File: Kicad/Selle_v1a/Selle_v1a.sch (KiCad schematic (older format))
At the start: 13 parts

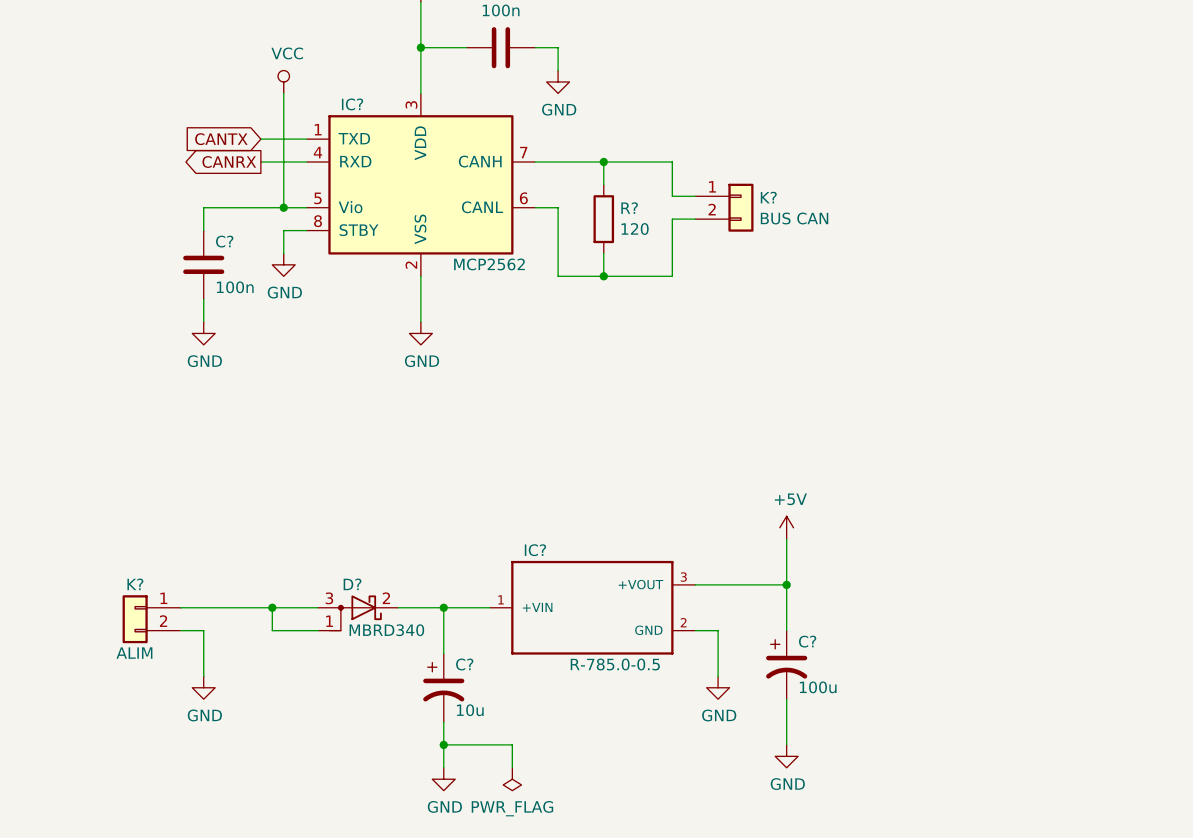
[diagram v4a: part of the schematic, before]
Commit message: Update
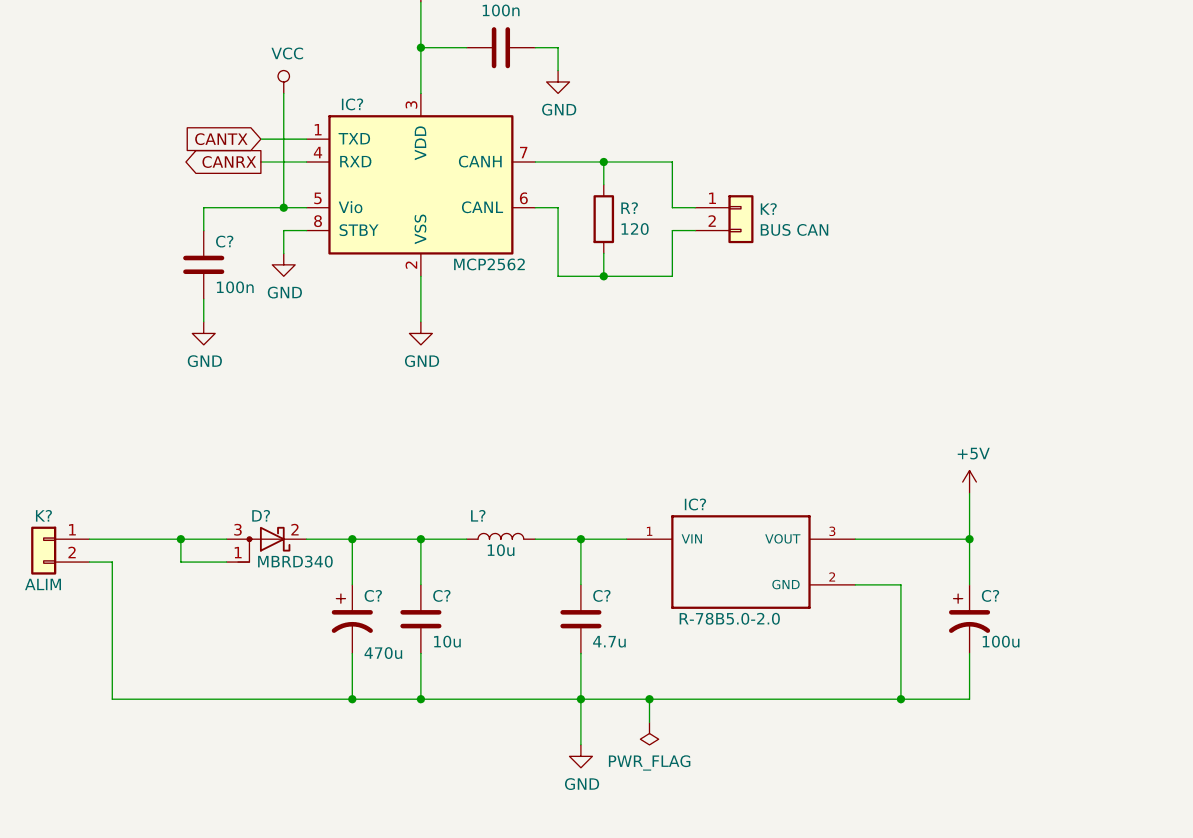
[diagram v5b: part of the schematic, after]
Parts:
- removed C?: 10u, symbol Device:CP1
- removed IC?: R-785.0-0.5, RECOM_R-785.0-0.5, symbol R-785.0-0.5:R-785.0-0.5
- added C?: 4.7u, symbol Device:C
- added C?: 10u, symbol Device:C
- added C?: 470u, symbol Device:CP1
- added IC?: R-78B5.0-2.0, CONV_R-78B15-2.0, symbol R-78B15-2.0:R-78B15-2.0
- added L?: 10u, symbol Device:L
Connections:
- net +5V: now also IC?.3 (VOUT)
- net GND: now also C?.2, C?.2, C?.2, IC?.2 (GND)
- net at D?.2 (K): now also C?.1, C?.1, L?.1
- new net: C?.1, IC?.1 (VIN), L?.2
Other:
- moved on the sheet: C?, D?, K?

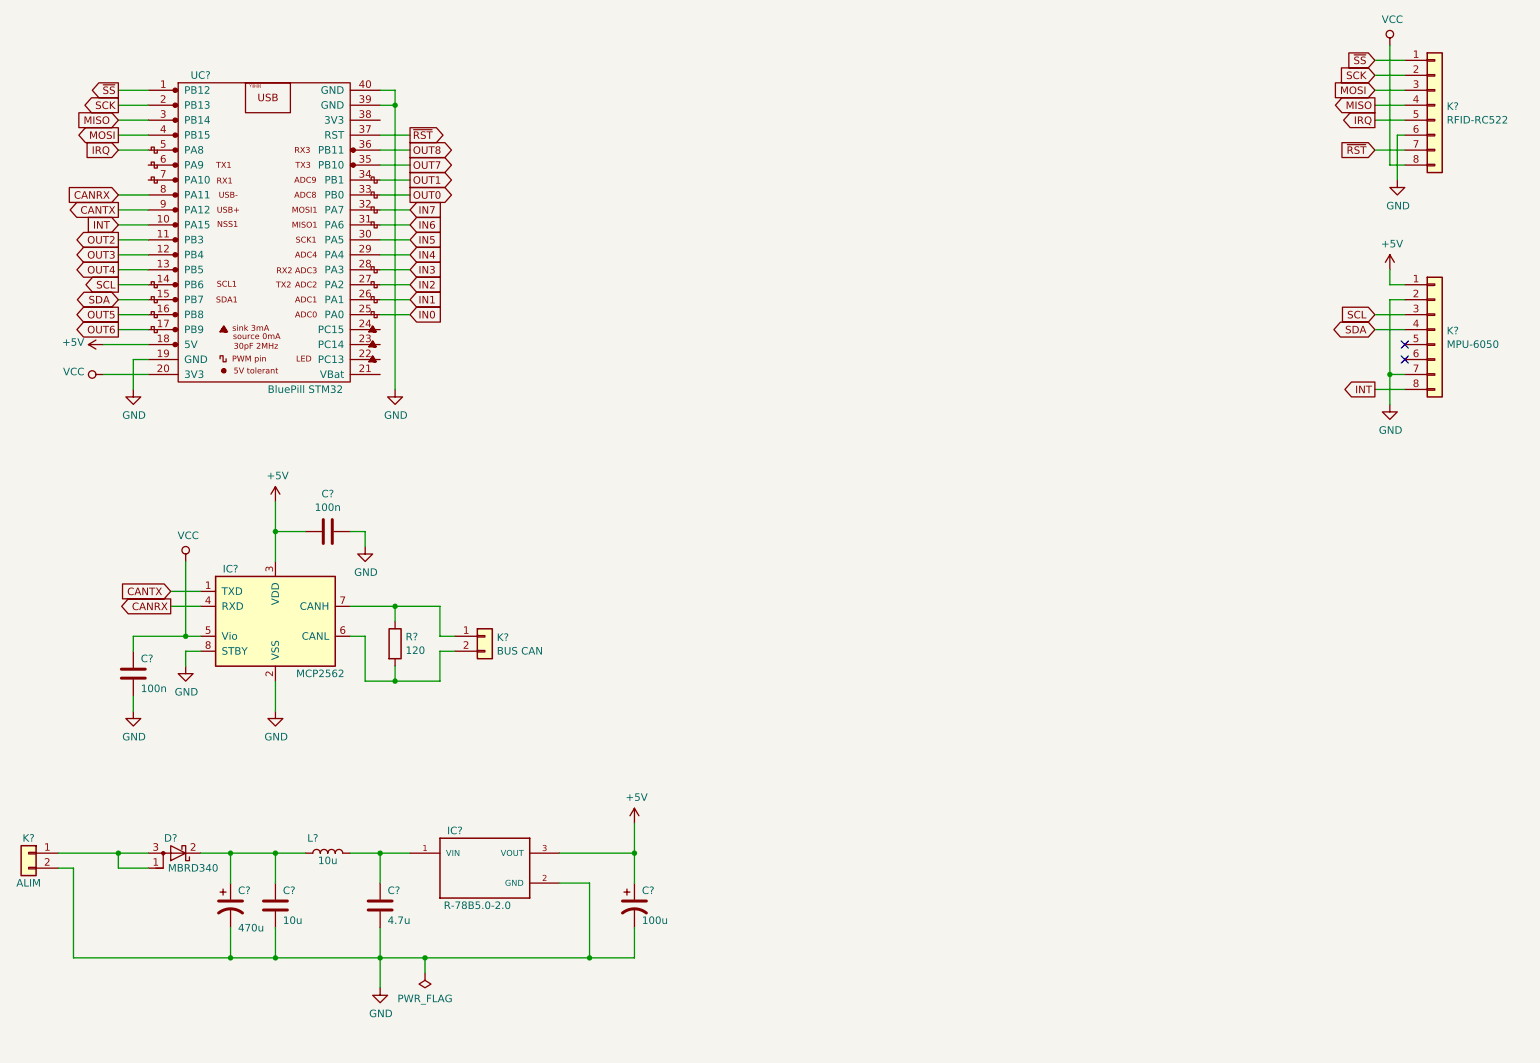
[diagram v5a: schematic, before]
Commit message: Update
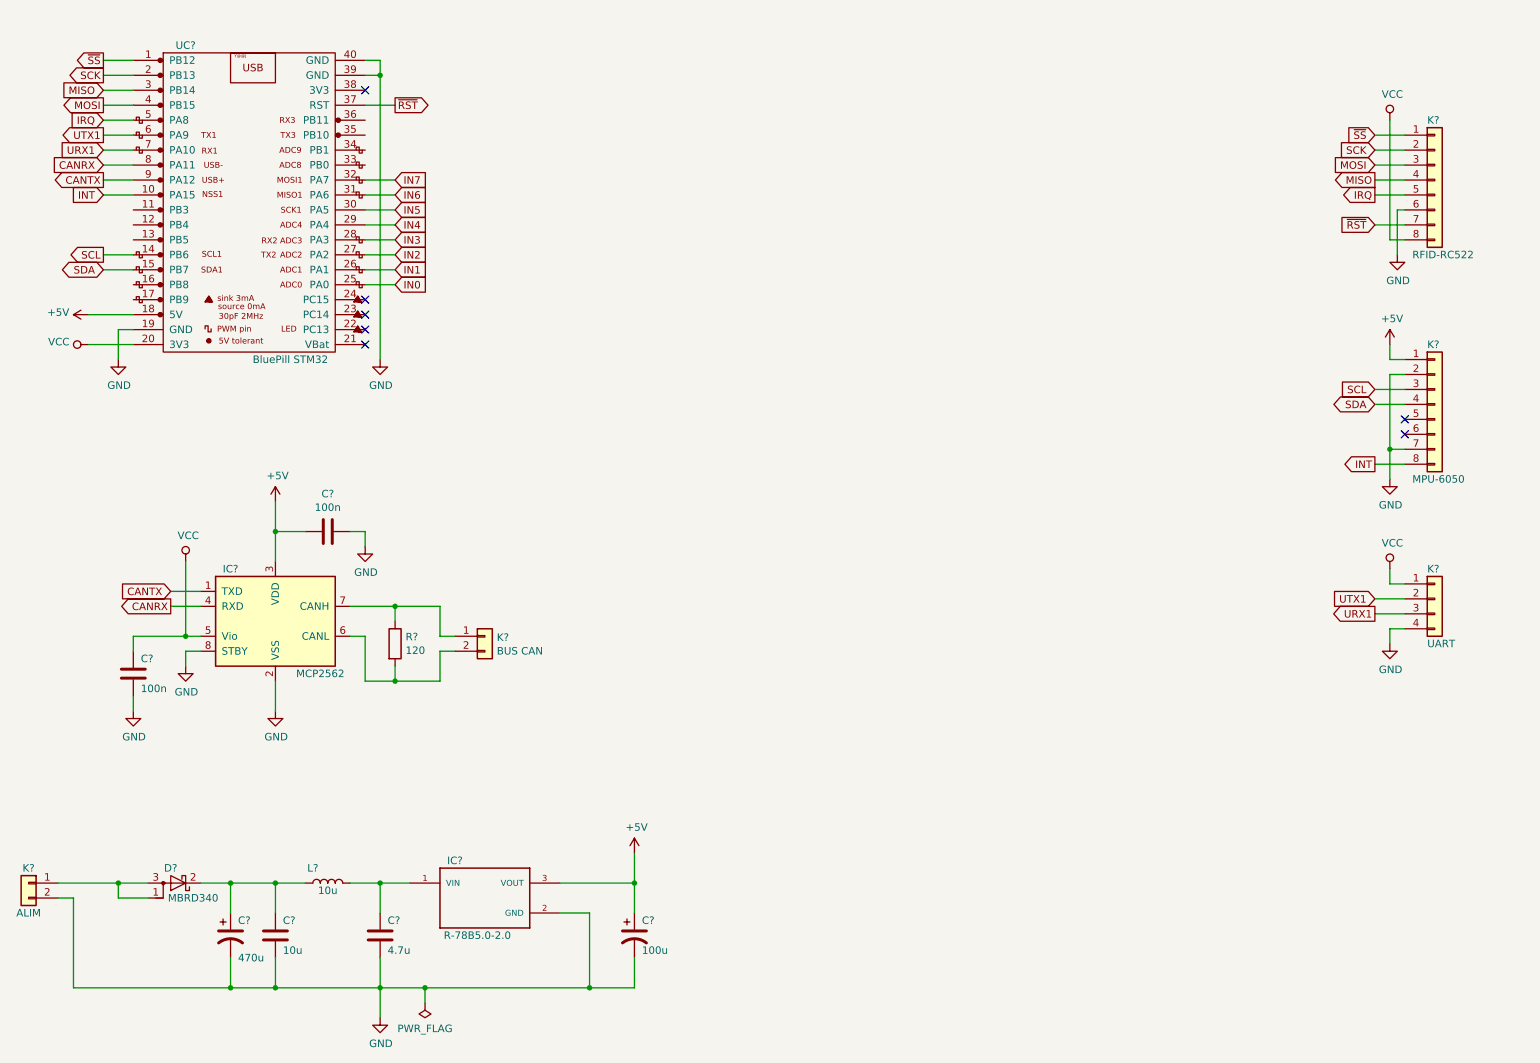
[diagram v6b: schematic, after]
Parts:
- added K?: UART, symbol Connector_Generic:Conn_01x04
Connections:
- net GND: now also K?.4 (Pin_4)
- net VCC: now also K?.1 (Pin_1)
- net UTX1: now reaches UC?.6 (PA9)
- net UTX1: now also K?.2 (Pin_2)
- net URX1: now reaches UC?.7 (PA10)
- net URX1: now also K?.3 (Pin_3)
- net OUT0: no longer names the net of UC?.33 (PB0)
- net OUT1: no longer names the net of UC?.34 (PB1)
- net OUT2: no longer names the net of UC?.11 (PB3)
- net OUT3: no longer names the net of UC?.12 (PB4)
- net OUT4: no longer names the net of UC?.13 (PB5)
- net OUT5: no longer names the net of UC?.16 (PB8)
- net OUT6: no longer names the net of UC?.17 (PB9)
- net OUT7: no longer names the net of UC?.35 (PB10)
- net OUT8: no longer names the net of UC?.36 (PB11)
- no-connect marks 2 -> 7
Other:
- moved on the sheet: C?, D?, IC?, K?, L?, UC?

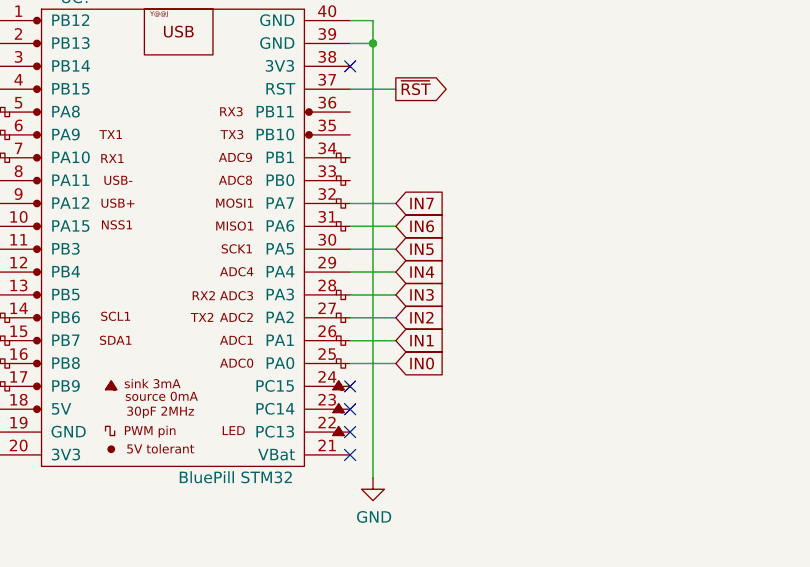
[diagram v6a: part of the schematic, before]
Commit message: Update
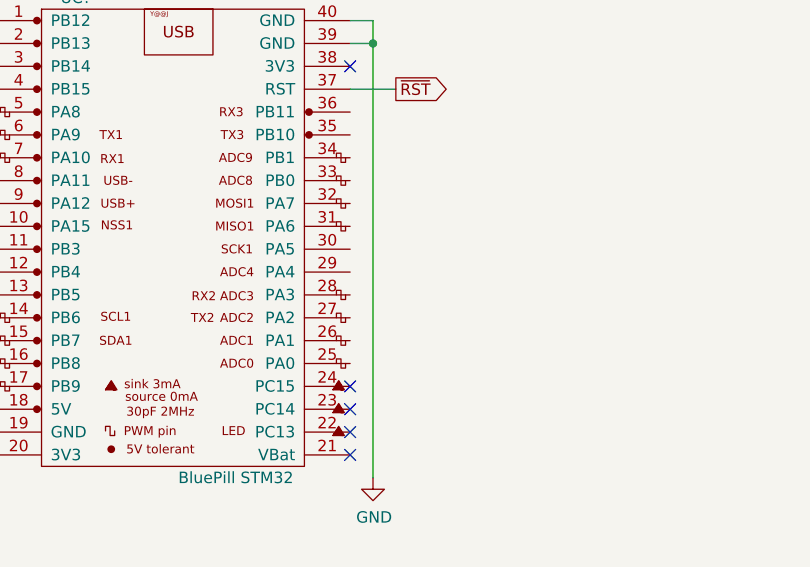
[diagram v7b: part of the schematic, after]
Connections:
- net IN0: no longer names the net of UC?.25 (PA0)
- net IN1: no longer names the net of UC?.26 (PA1)
- net IN2: no longer names the net of UC?.27 (PA2)
- net IN3: no longer names the net of UC?.28 (PA3)
- net IN4: no longer names the net of UC?.29 (PA4)
- net IN5: no longer names the net of UC?.30 (PA5)
- net IN6: no longer names the net of UC?.31 (PA6)
- net IN7: no longer names the net of UC?.32 (PA7)
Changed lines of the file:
@@
 NoConn ~ 3050 2900
 NoConn ~ 3050 1200
-Text GLabel 3250 1800 2    50   Input ~ 0
-IN7
-Text GLabel 3250 1900 2    50   Input ~ 0
-IN6
-Text GLabel 3250 2000 2    50   Input ~ 0
-IN5
-Text GLabel 3250 2100 2    50   Input ~ 0
-IN4
-Text GLabel 3250 2200 2    50   Input ~ 0
-IN3
-Text GLabel 3250 2300 2    50   Input ~ 0
-IN2
-Text GLabel 3250 2400 2    50   Input ~ 0
-IN1
-Text GLabel 3250 2500 2    50   Input ~ 0
-IN0
-Wire Wire Line
-	3050 1800 3250 1800
-Wire Wire Line
-	3050 1900 3250 1900
-Wire Wire Line
-	3050 2000 3250 2000
-Wire Wire Line
-	3050 2100 3250 2100
-Wire Wire Line
-	3050 2200 3250 2200
-Wire Wire Line
-	3050 2300 3250 2300
-Wire Wire Line
-	3050 2400 3250 2400
-Wire Wire Line
-	3050 2500 3250 2500
 $EndSCHEMATC
